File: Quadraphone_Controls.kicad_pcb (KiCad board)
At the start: 2 copper layers, 60 x 110 mm, 17 parts, among them J1 Conn_01x10_Female, J10 Pitch_In, J11 Mix_Out, J2 Conn_01x10_Female, J3 Conn_01x10_Female, J4 Conn_01x10_Female, J5 PWM_CV, J6 LFO_IN, J7 PWM_CV_In, J8 Synch_Signal_In, J9 Freq_Mod_In, SW1 Synch_Type, SW2 Output_Type

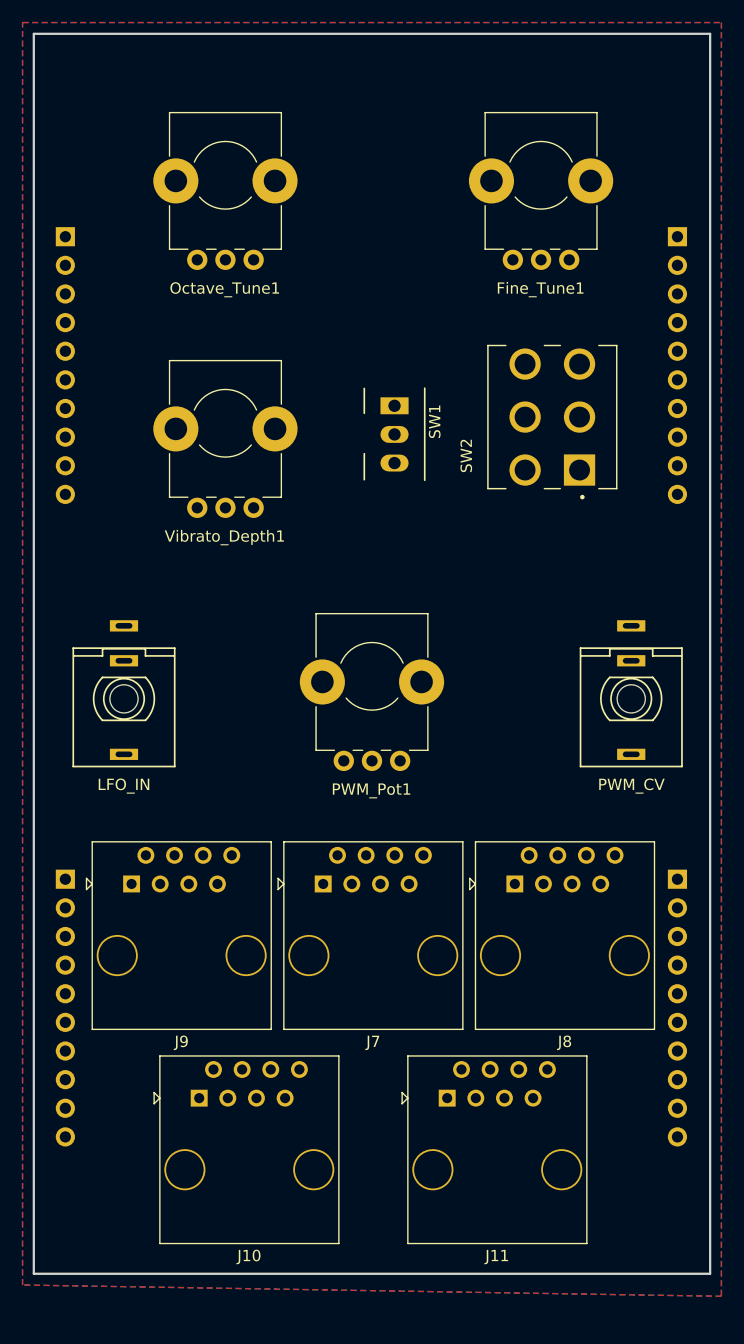
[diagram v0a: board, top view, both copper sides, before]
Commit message: Started laying out Panel
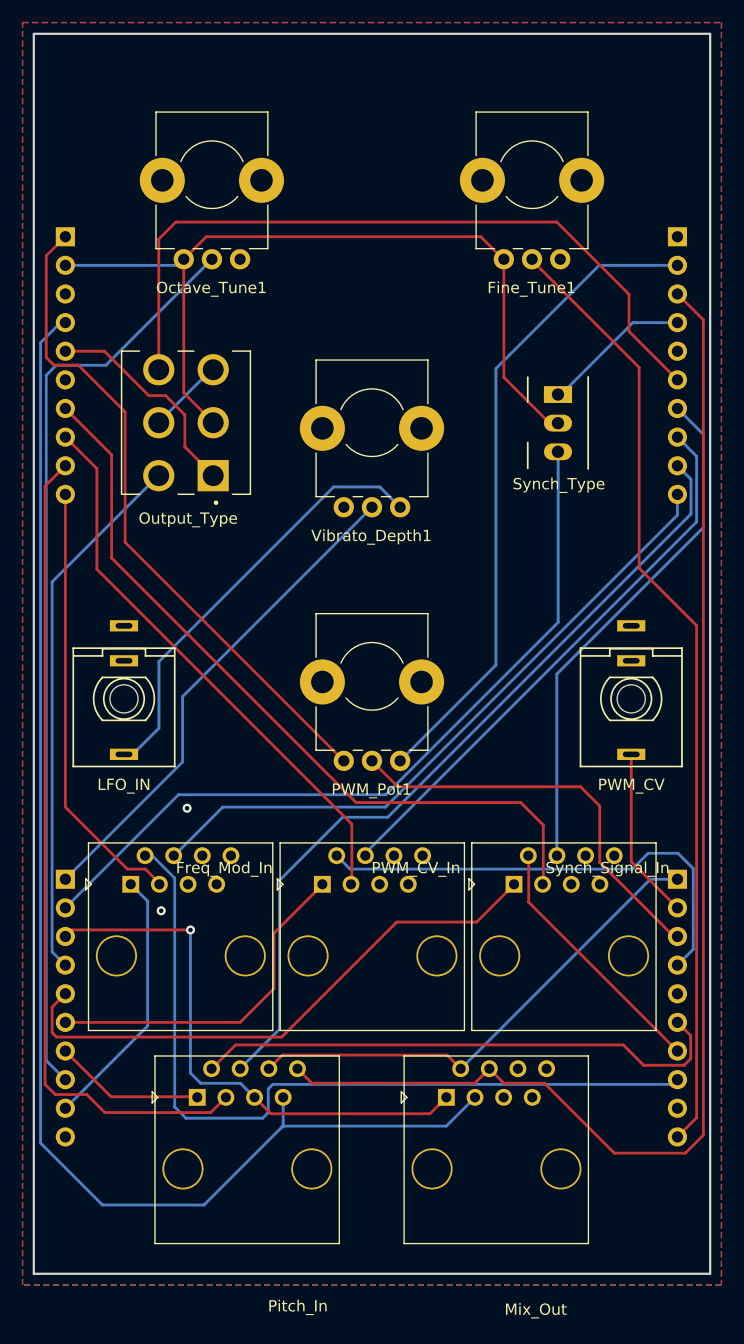
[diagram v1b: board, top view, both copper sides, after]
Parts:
- moved SW2 32.5 mm to (63.5, 79.5)
- moved SW1 14.5 mm to (96.5, 77.0)
- moved Vibrato_Depth1 13.0 mm to (80.0, 79.5)
- moved J7 6.37 mm to (80.0, 125.1)
- moved J8 6.37 mm to (97.0, 125.1)
- moved J9 6.37 mm to (63.0, 125.1)
- moved J11 6.30 mm to (91.0, 144.0)
- moved J10 6.23 mm to (68.9, 144.0)
- moved Octave_Tune1 1.20 mm to (65.8, 57.5)
- moved Fine_Tune1 0.80 mm to (94.2, 57.5)
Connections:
- Fine_Tune1 pad 3: +2V5 -> +5V
- J3 pad 10: /OCT_TUNE -> /FINE_TUNE
- J4 pad 8: /FINE_TUNE -> /OCT_TUNE
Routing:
- net /MIX_OUT2: track 0.00 -> 121.6 mm
- net /MIX_OUT1: track 0.00 -> 116.4 mm
- net /FINE_TUNE: track 0.00 -> 84.6 mm
- net /OCT_TUNE: track 0.00 -> 82.2 mm
- net +5V: track 0.00 -> 73.4 mm
- net /V_PER_OCT2: track 0.00 -> 73.3 mm
- net /V_PER_OCT1: track 0.00 -> 73.1 mm
- net /FREQ_MOD3: track 0.00 -> 71.5 mm
- net /SOFT_SYNCH_SW: track 0.00 -> 69.1 mm
- net /SYNCH_SIGNAL2: track 0.00 -> 68.3 mm
- net /SAW_SW: track 0.00 -> 65.9 mm
- net +12V: track 0.00 -> 59.4 mm
- net /FREQ_MOD1: track 0.00 -> 59.0 mm
- net -12V: track 0.00 -> 58.2 mm
- net /SYNCH_SIGNAL4: track 0.00 -> 50.7 mm
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- added copper zone on B.Cu, net GND
- added copper zone on F.Cu, net GND
- removed copper zone on B.Cu, net (none)
- removed copper zone on F.Cu, net (none)
